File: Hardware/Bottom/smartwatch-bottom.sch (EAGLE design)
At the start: 31 parts, among them U2 AD5242-SO16

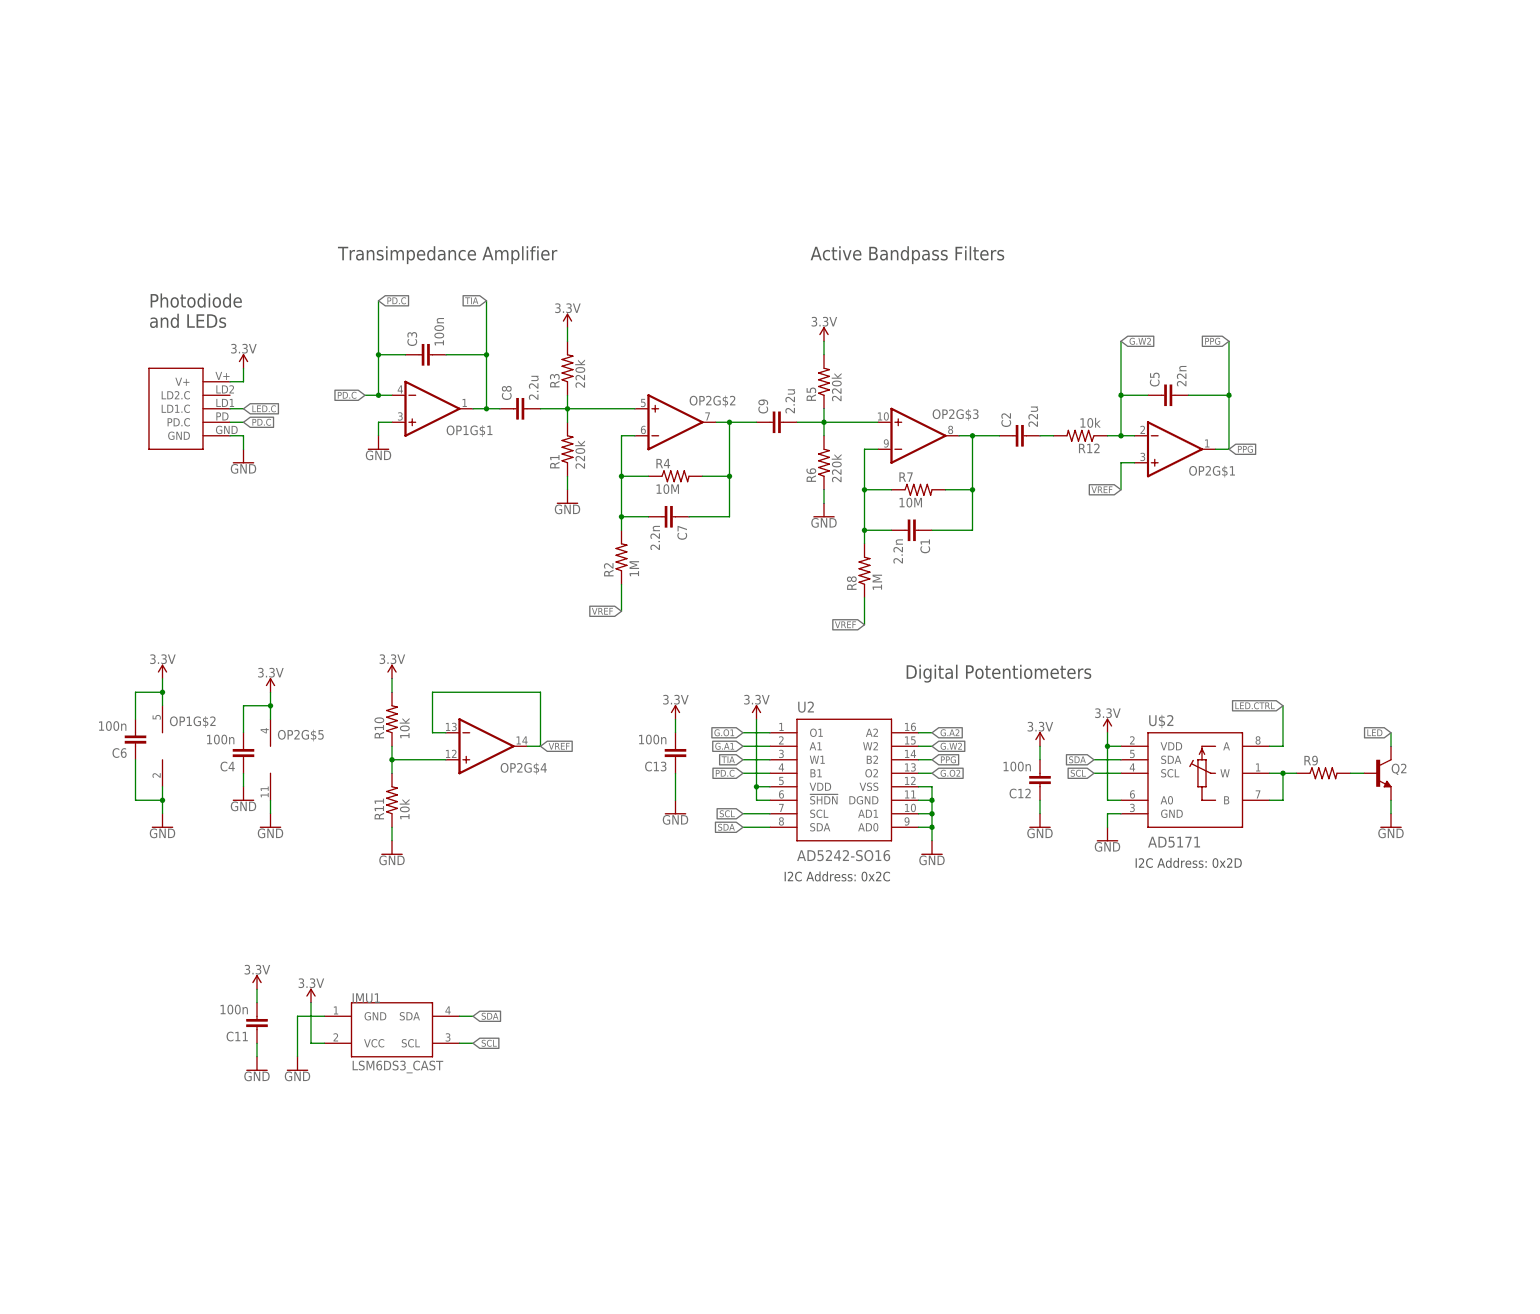
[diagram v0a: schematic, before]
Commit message: Finished Take003
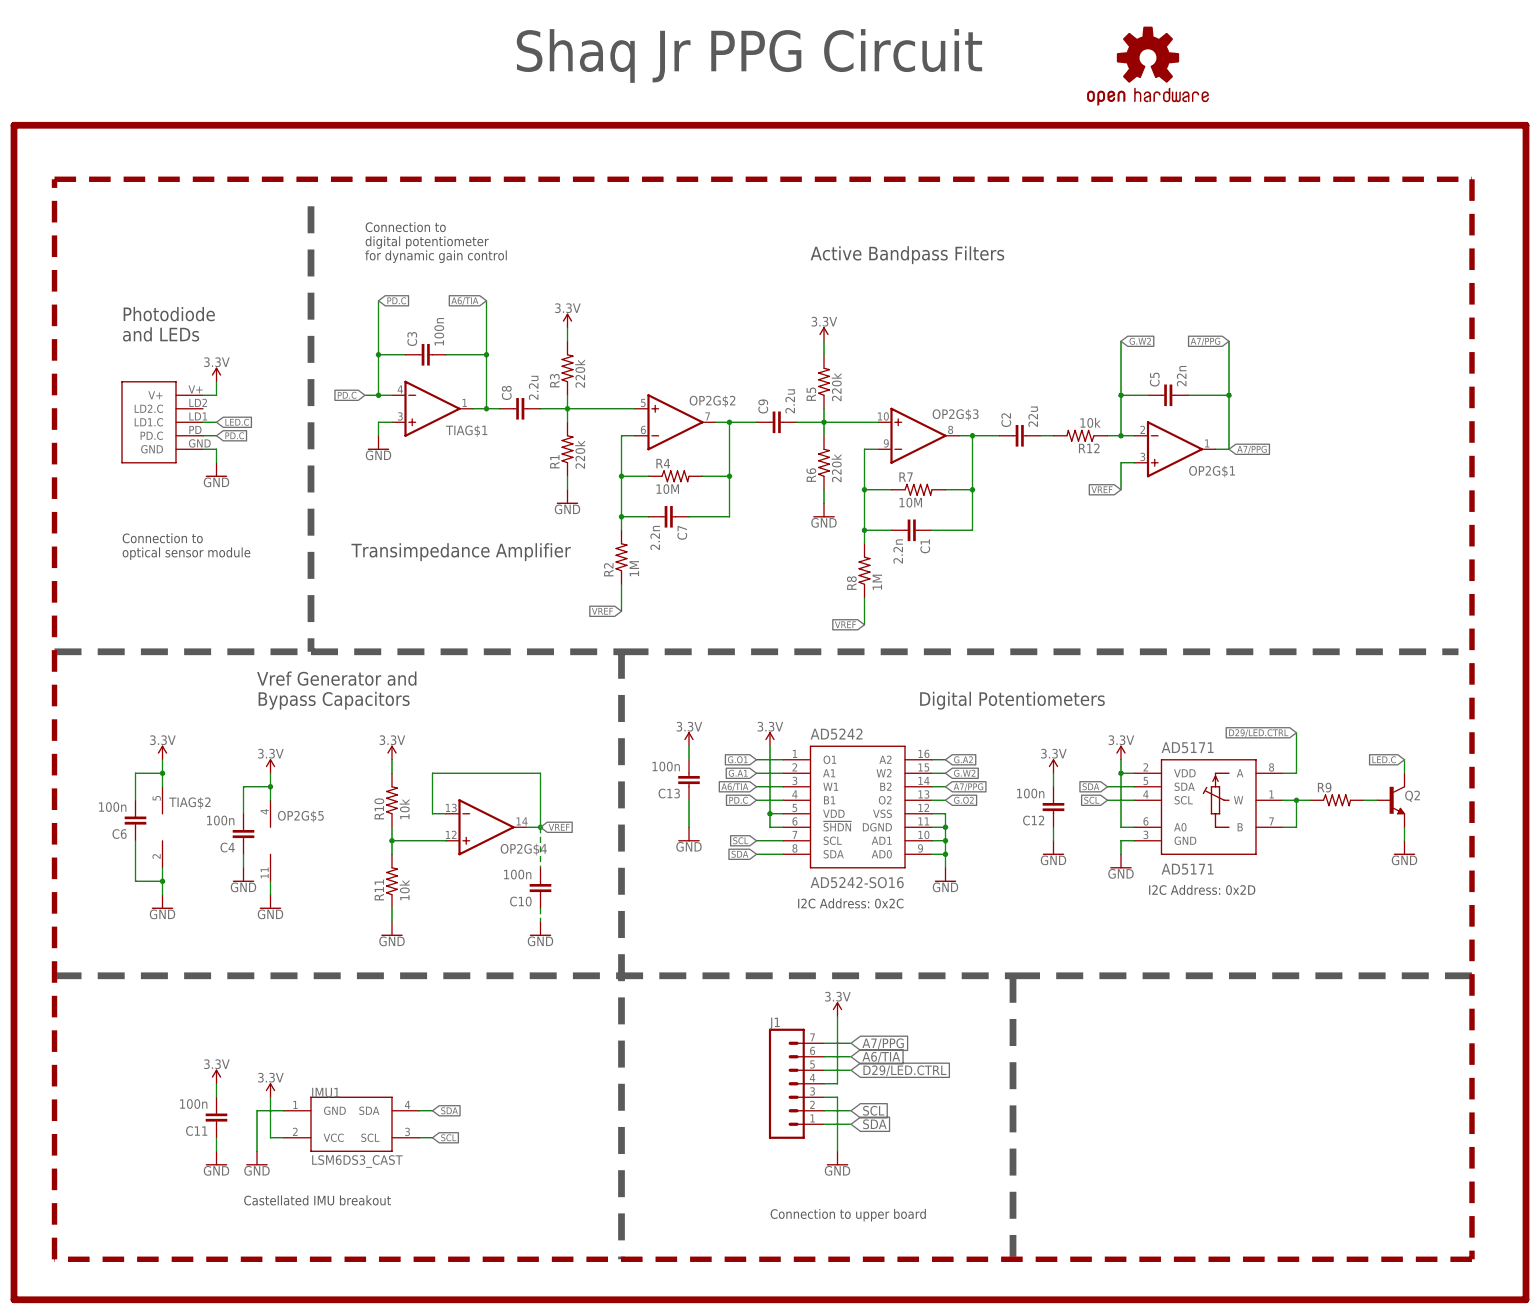
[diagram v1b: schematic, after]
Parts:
- removed U$2: AD5171, LinnesLab-DigitalIC:AD5171
- removed U2: AD5242-SO16, LinnesLab-DigitalIC:AD5242-SO16
- added AD5171: AD5171, LinnesLab-DigitalIC:AD5171
- added AD5242: AD5242-SO16, LinnesLab-DigitalIC:AD5242-SO16
- added C10: 100n, LinnesLab-Passives:CAPACITOR0603
- added J1: (no value), LinnesLab-Connectors:CONN_07-1.27MM
- added LOGO1: REVISION.A, LinnesLab-Logos:REVISION.A
- added LOGO2: OSHW-LOGOS, LinnesLab-Logos:OSHW-LOGOS
- renumbered OP1 to TIA
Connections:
- removed net LED: Q2.C
- removed net LED.CTRL: U$2.A
- removed net PPG: C5.2, OP2G$1.OUT, U2.B2
- removed net TIA: C3.2, C8.1, TIAG$1.OUT, U2.W1
- new net A6/TIA: AD5242.W1, C3.2, C8.1, J1.6, TIAG$1.OUT
- new net A7/PPG: AD5242.B2, C5.2, J1.7, OP2G$1.OUT
- new net D29/LED.CTRL: AD5171.A, J1.5
- net 3.3V: now also AD5171.A0, AD5171.VDD, AD5242.!SHDN, AD5242.VDD, J1.4; no longer U$2.A0, U$2.VDD, U2.!SHDN, U2.VDD
- net G.A1: now also AD5242.A1; no longer U2.A1
- net G.A2: now also AD5242.A2; no longer U2.A2
- net G.O1: now also AD5242.O1; no longer U2.O1
- net G.O2: now also AD5242.O2; no longer U2.O2
- net G.W2: now also AD5242.W2; no longer U2.W2
- net GND: now also AD5171.GND, AD5242.AD0, AD5242.AD1, AD5242.DGND, AD5242.VSS, C10.1, J1.3; no longer U$2.GND, U2.AD0, U2.AD1, U2.DGND, U2.VSS
- net LED.C: now also Q2.C
- net N$12: now also AD5171.B, AD5171.W; no longer U$2.B, U$2.W
- net PD.C: now also AD5242.B1; no longer U2.B1
- net SCL: now also AD5171.SCL, AD5242.SCL, J1.2; no longer U$2.SCL, U2.SCL
- net SDA: now also AD5171.SDA, AD5242.SDA, J1.1; no longer U$2.SDA, U2.SDA
- net VREF: now also C10.2
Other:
- note added: "Castellated IMU breakout"
- note added: "Connection to digital potentiometer for dynamic gain control"
- note added: "Connection to optical sensor module"
- note added: "Connection to upper board"
- note added: "Shaq Jr PPG Circuit"
- note added: "Vref Generator and Bypass Capacitors"
- moved on the sheet: C11, C12, C13, C4, C6, IMU1, OP2G$4, OP2G$5, Q2, R10, R11, R9
